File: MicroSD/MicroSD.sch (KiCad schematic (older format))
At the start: 15 parts, among them J1 Conn_01x04, J2 Conn_01x04, J3 Micro_SD_Card_Det, U1 AP7365, U2 4050

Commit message: Part Numbers Added
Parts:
- C1, C2: Part (none) -> C29936
- D1: Part (none) -> C118330
- J3: Part (none) -> C114218
- R1: Part (none) -> C227816
- R3: Part (none) -> C99198
- R6: Part (none) -> C25585
- U1: Part (none) -> C264087
- U2: Part (none) -> C352821
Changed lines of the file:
@@
 F 2 "Connector_Card:microSD_HC_Hirose_DM3AT-SF-PEJM5" H 8850 4450 50  0001 C CNN
 F 3 "https://www.hirose.com/product/en/download_file/key_name/DM3/category/Catalog/doc_file_id/49662/?file_category_id=4&item_id=195&is_series=1" H 6800 3850 50  0001 C CNN
+F 4 "C114218" H 6800 3750 50  0001 C CNN "Part"
 	1    6800 3750
 	1    0    0    -1
@@
 F 2 "Package_SO:SOIC-16_3.9x9.9mm_P1.27mm" H 2500 4550 50  0001 C CNN
 F 3 "http://www.intersil.com/content/dam/intersil/documents/cd40/cd4050bms.pdf" H 2500 4550 50  0001 C CNN
+F 4 "C352821" H 2500 4550 50  0001 C CNN "Part"
 	7    2500 4550
 	1    0    0    -1
@@
 F 2 "Package_TO_SOT_SMD:SOT-23-5" H 9300 4250 50  0001 C CNN
 F 3 "" H 9300 4250 50  0001 C CNN
+F 4 "C264087" H 9250 3250 50  0001 C CNN "Part"
 	1    9250 3250
 	1    0    0    -1
@@
 F 2 "Capacitor_SMD:C_0603_1608Metric" H 8688 2650 50  0001 C CNN
 F 3 "~" H 8650 2800 50  0001 C CNN
+F 4 "C29936" H 8650 2800 50  0001 C CNN "Part"
 	1    8650 2800
 	1    0    0    -1
@@
 F 2 "Capacitor_SMD:C_0603_1608Metric" H 9938 2650 50  0001 C CNN
 F 3 "~" H 9900 2800 50  0001 C CNN
+F 4 "C29936" H 9900 2800 50  0001 C CNN "Part"
 	1    9900 2800
 	1    0    0    -1
@@
 F 2 "Resistor_SMD:R_0603_1608Metric" V 9440 4240 50  0001 C CNN
 F 3 "~" H 9400 4250 50  0001 C CNN
+F 4 "C227816" H 9400 4250 50  0001 C CNN "Part"
 	1    9400 4250
 	1    0    0    -1
@@
 F 2 "Resistor_SMD:R_0603_1608Metric" V 9440 4840 50  0001 C CNN
 F 3 "~" H 9400 4850 50  0001 C CNN
+F 4 "C99198" H 9400 4850 50  0001 C CNN "Part"
 	1    9400 4850
 	1    0    0    -1
@@
 F 2 "Resistor_SMD:R_0603_1608Metric" V 4790 4790 50  0001 C CNN
 F 3 "~" H 4750 4800 50  0001 C CNN
+F 4 "C25585" V 4750 4800 50  0001 C CNN "Part"
 	1    4750 4800
 	0    -1   -1   0
@@
 F 2 "LED_SMD:LED_0603_1608Metric" H 5150 4800 50  0001 C CNN
 F 3 "~" H 5150 4800 50  0001 C CNN
+F 4 "C118330" H 5150 4800 50  0001 C CNN "Part"
 	1    5150 4800
 	-1   0    0    1

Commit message: MicroSDv2 Removed and MicroSD and MicroSD_DualVoltage Updated
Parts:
- removed J1, J2: Conn_01x04, Connector_PinHeader_2.54mm:PinHeader_1x04_P2.54mm_Vertical, symbol Connector_Generic:Conn_01x04
- added J1: Conn_01x08, Connector_PinHeader_2.54mm:PinHeader_1x08_P2.54mm_Vertical, symbol Connector_Generic:Conn_01x08
- U1: Part C264087 -> (none)
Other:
- moved on the sheet: C1, C2, D1, H1, H2, H3, H4, J3, R1, R3, R6, U1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

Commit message: Schematic PDF and 3D Renders added
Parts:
- U1: symbol U.FL-R-SMT(01):AP7365 -> MicroSD-rescue:AP7365-U.FL-R-SMT(01)
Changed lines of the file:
@@
 EESchema Schematic File Version 4
-LIBS:MicroSDv2-cache
+LIBS:MicroSD-cache
 EELAYER 29 0
 EELAYER END
@@
 $EndComp
 $Comp
-L U.FL-R-SMT(01):AP7365 U1
+L MicroSD-rescue:AP7365-U.FL-R-SMT(01) U1
 U 1 1 5DB62551
 P 8425 5775

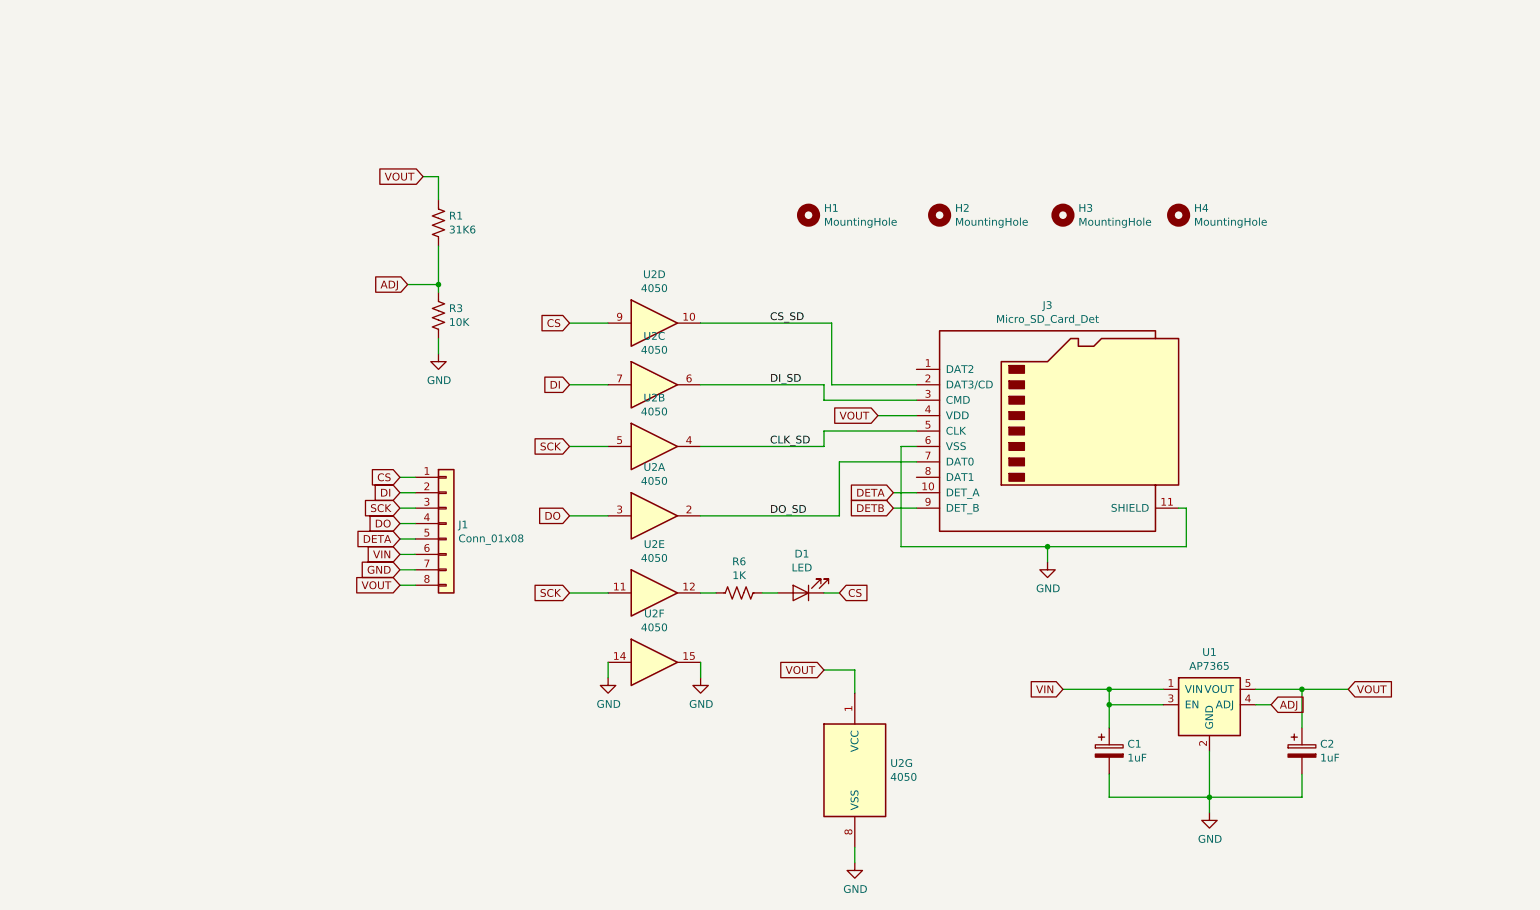
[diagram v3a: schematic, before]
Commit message: Board Redesign
Revision3
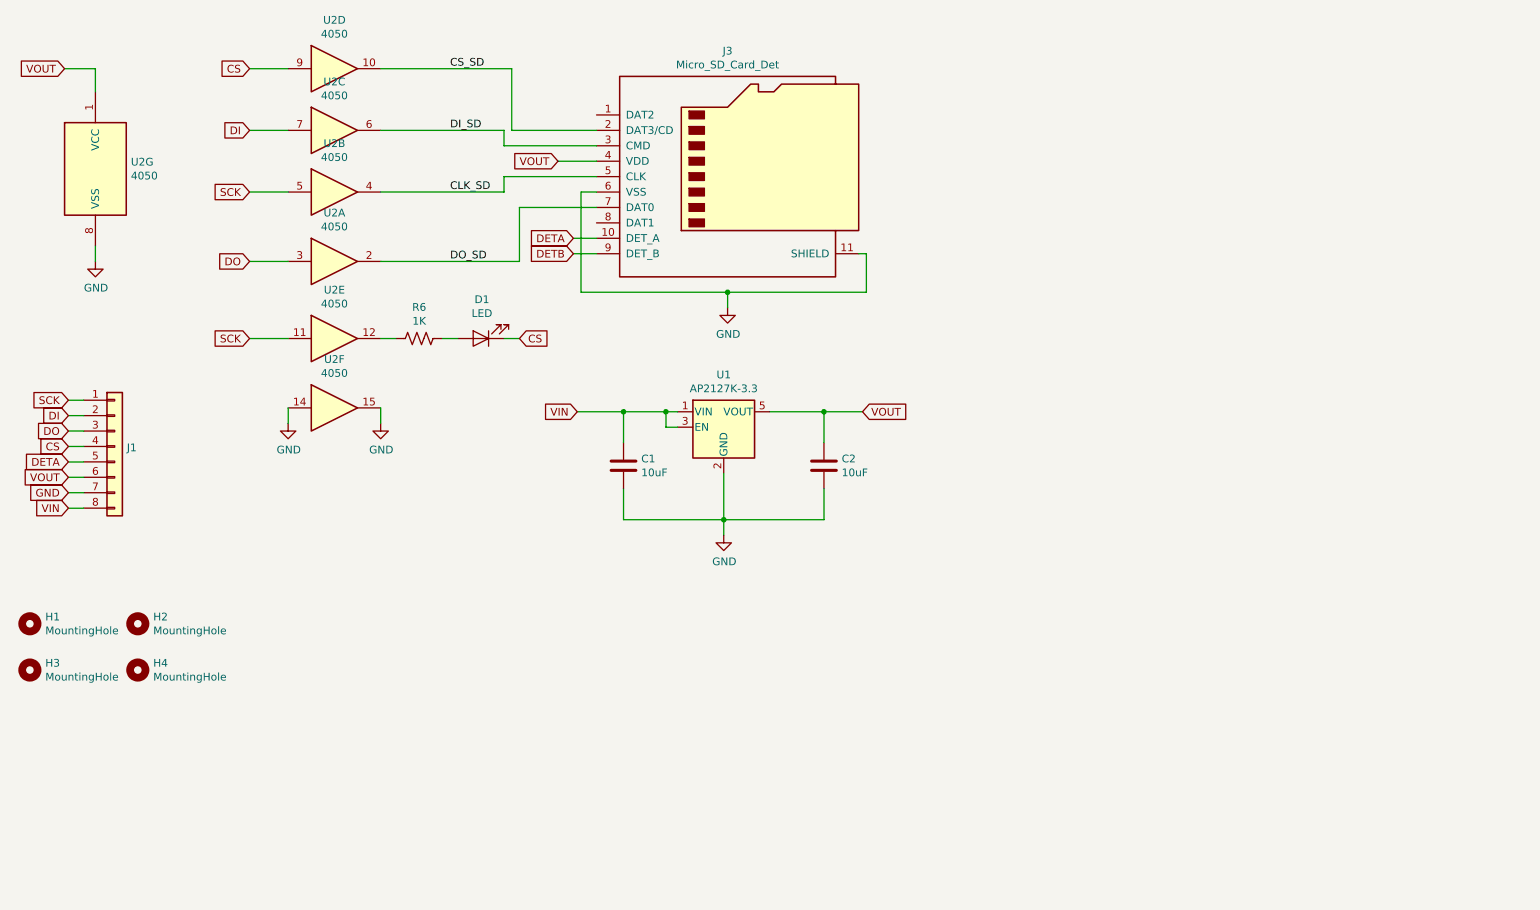
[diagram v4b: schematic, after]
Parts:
- removed C1, C2: 1uF, Capacitor_SMD:C_0603_1608Metric, symbol Device:CP
- removed R1: 31K6, Resistor_SMD:R_0603_1608Metric, symbol Device:R_US
- removed R3: 10K, Resistor_SMD:R_0603_1608Metric, symbol Device:R_US
- removed U1: AP7365, Package_TO_SOT_SMD:SOT-23-5, symbol MicroSD-rescue:AP7365-U.FL-R-SMT(01)
- added C1, C2: 10uF, Capacitor_SMD:C_0805_2012Metric, symbol Device:C
- added U1: AP2127K-3.3, Package_TO_SOT_SMD:SOT-23-5, symbol Regulator_Linear:AP2127K-3.3
- H1, H2, H3, H4: footprint MountingHole:MountingHole_2.7mm_M2.5_ISO14580_Pad -> SirBoardLibrary:MountingHole_M2.5_SirBoard
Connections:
- net CS: now also J1.4 (Pin_4); no longer J1.1 (Pin_1)
- net DO: now also J1.3 (Pin_3); no longer J1.4 (Pin_4)
- net GND: now also C1.2, C2.2, U1.2 (GND)
- net SCK: now also J1.1 (Pin_1); no longer J1.3 (Pin_3)
- net VIN: now also J1.8 (Pin_8), C1.1, U1.1 (VIN), U1.3 (EN); no longer J1.6 (Pin_6)
- net VOUT: now also J1.6 (Pin_6), C2.1, U1.5 (VOUT); no longer J1.8 (Pin_8)
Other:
- moved on the sheet: D1, H1, J1, J3, R6, U2A, U2B, U2C, U2D, U2E, U2F, U2G
